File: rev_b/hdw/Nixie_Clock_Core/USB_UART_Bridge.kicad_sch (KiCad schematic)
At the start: 34 parts, among them J1301 USB_B_Mini, U1301 TLV6700, U1302 FT234XD, U1304 TXB0102DCU, U1305 TPD3S014DBVR

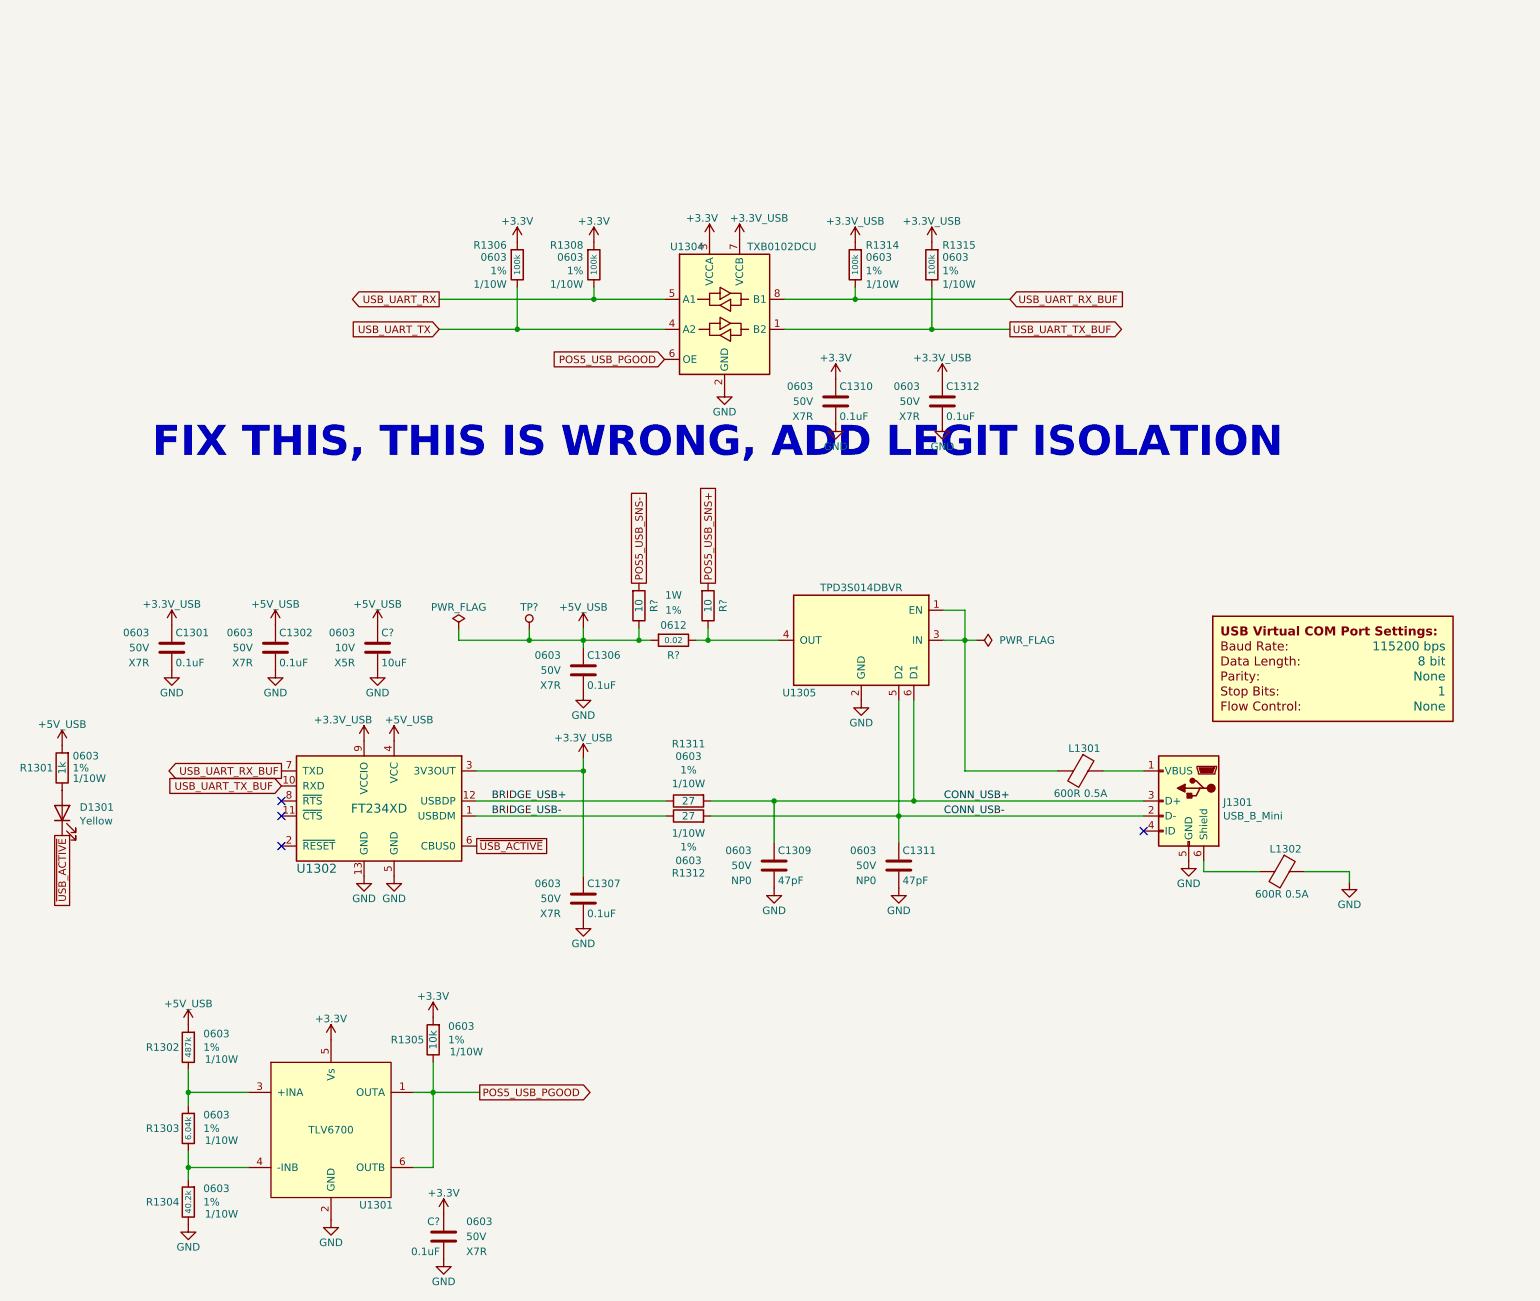
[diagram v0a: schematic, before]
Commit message: lots of rev B control board schematic progress
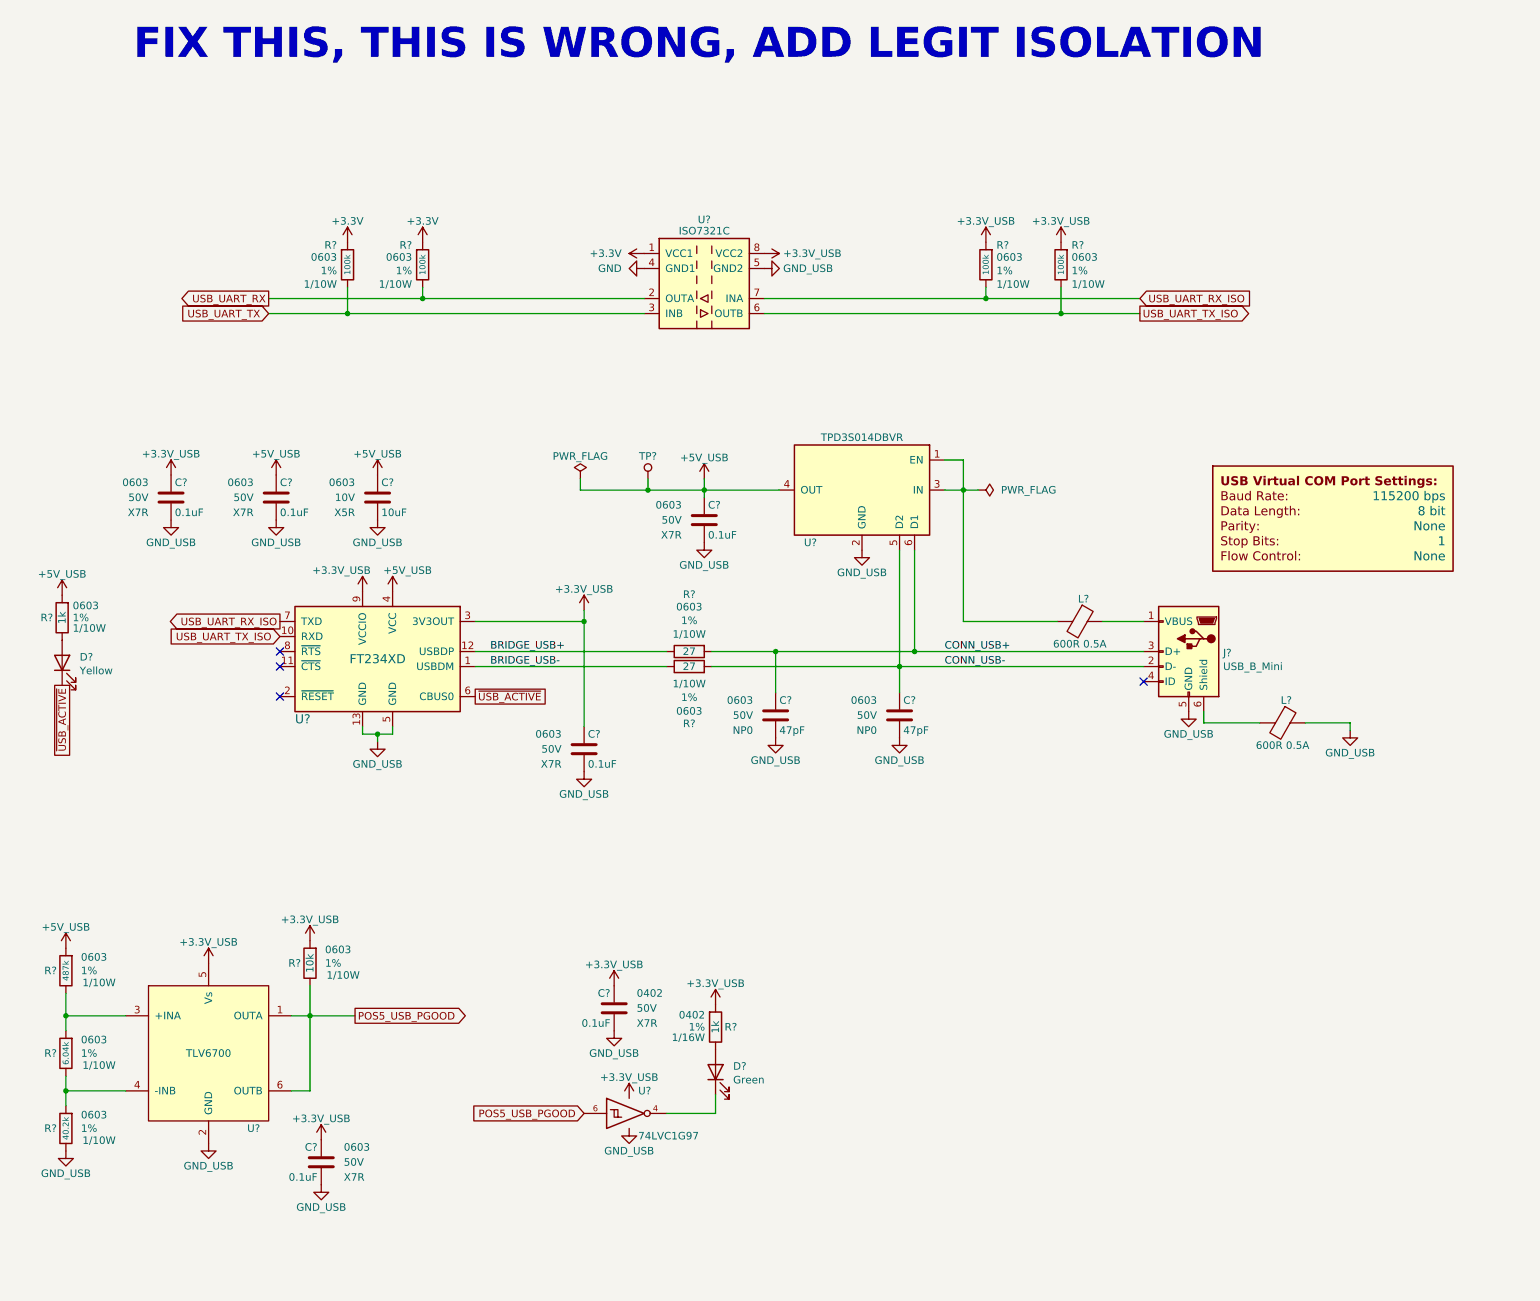
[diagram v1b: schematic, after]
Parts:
- removed C1310, C1312: 0.1uF, Capacitors_SMD:C_0603, symbol Custom_Library:C_Custom
- removed R? (x2): 10, Resistors_SMD:R_0603, symbol Custom_Library:R_Custom
- removed R?: 0.02, Resistors_SMD:R_0612, symbol Custom_Library:R_Custom
- removed U1304: TXB0102DCU, Package_SO:VSSOP-8_2.4x2.1mm_P0.5mm, symbol Logic_LevelTranslator:TXB0102DCU
- added C?: 0.1uF, Capacitors_SMD:C_0402, symbol Custom_Library:C_Custom
- added D?: Green, LEDs:LED_0402, symbol Device:LED
- added R?: 1k, Resistors_SMD:R_0402, symbol Custom_Library:R_Custom
- added U?: 74LVC1G97, Package_TO_SOT_SMD:SOT-363_SC-70-6, symbol Custom Library:74LVC1G97_Power_NOT
- added U?: ISO7321C, Package_SO:SOIC-8_3.9x4.9mm_P1.27mm, symbol Isolator:ISO7321C
- renumbered C1307 to C?, C1309 to C?, C1311 to C?, C1302 to C?, C1306 to C?, C1301 to C?, D1301 to D?, DOC1301 to DOC?, J1301 to J?, L1301 to L?, L1302 to L?, R1314 to R?, R1312 to R?, R1302 to R?, R1311 to R?, R1305 to R?, R1315 to R?, R1304 to R?, R1301 to R?, R1306 to R?, R1303 to R?, R1308 to R?, U1302 to U?, U1301 to U?, U1305 to U?
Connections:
- net +3.3V: now also U?.1 (VCC1); no longer C?.1, R?.1, U?.5 (Vs)
- net +3.3V_USB: now also C?.1, R?.1, U?.5 (Vs), C?.1, R?.1, U?.1 (VCC), U?.5 (VCC), U?.8 (VCC2)
- net +5V_USB: now also U?.4 (OUT)
- net GND: now also U?.4 (GND1); no longer C?.2, C?.2, C?.2, C?.2, C?.2, C?.2, C?.2, C?.2, J?.5 (GND), L?.1, R?.2, U?.13 (GND), U?.2 (GND), U?.2 (GND), U?.5 (GND)
- net POS5_USB_PGOOD: now also U?.6
- net USB_UART_RX: now also U?.2 (OUTA)
- net USB_UART_TX: now also U?.3 (INB)
- net USB_UART_RX_BUF renamed USB_UART_RX_ISO
- net USB_UART_RX_ISO: now also U?.7 (INA)
- net USB_UART_TX_BUF renamed USB_UART_TX_ISO
- net USB_UART_TX_ISO: now also U?.6 (OUTB)
- new net: D?.1 (K), U?.4
- new net: D?.2 (A), R?.2
- new net GND_USB: C?.2, C?.2, C?.2, C?.2, C?.2, C?.2, C?.2, C?.2, C?.2, J?.5 (GND), L?.1, R?.2, U?.13 (GND), U?.2 (GND), U?.2 (GND), U?.2 (GND), U?.3 (GND), U?.5 (GND), U?.5 (GND2)
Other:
- moved on the sheet: C?, D?, J?, L?, R?, TP?, U?

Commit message: more rev b sch progress
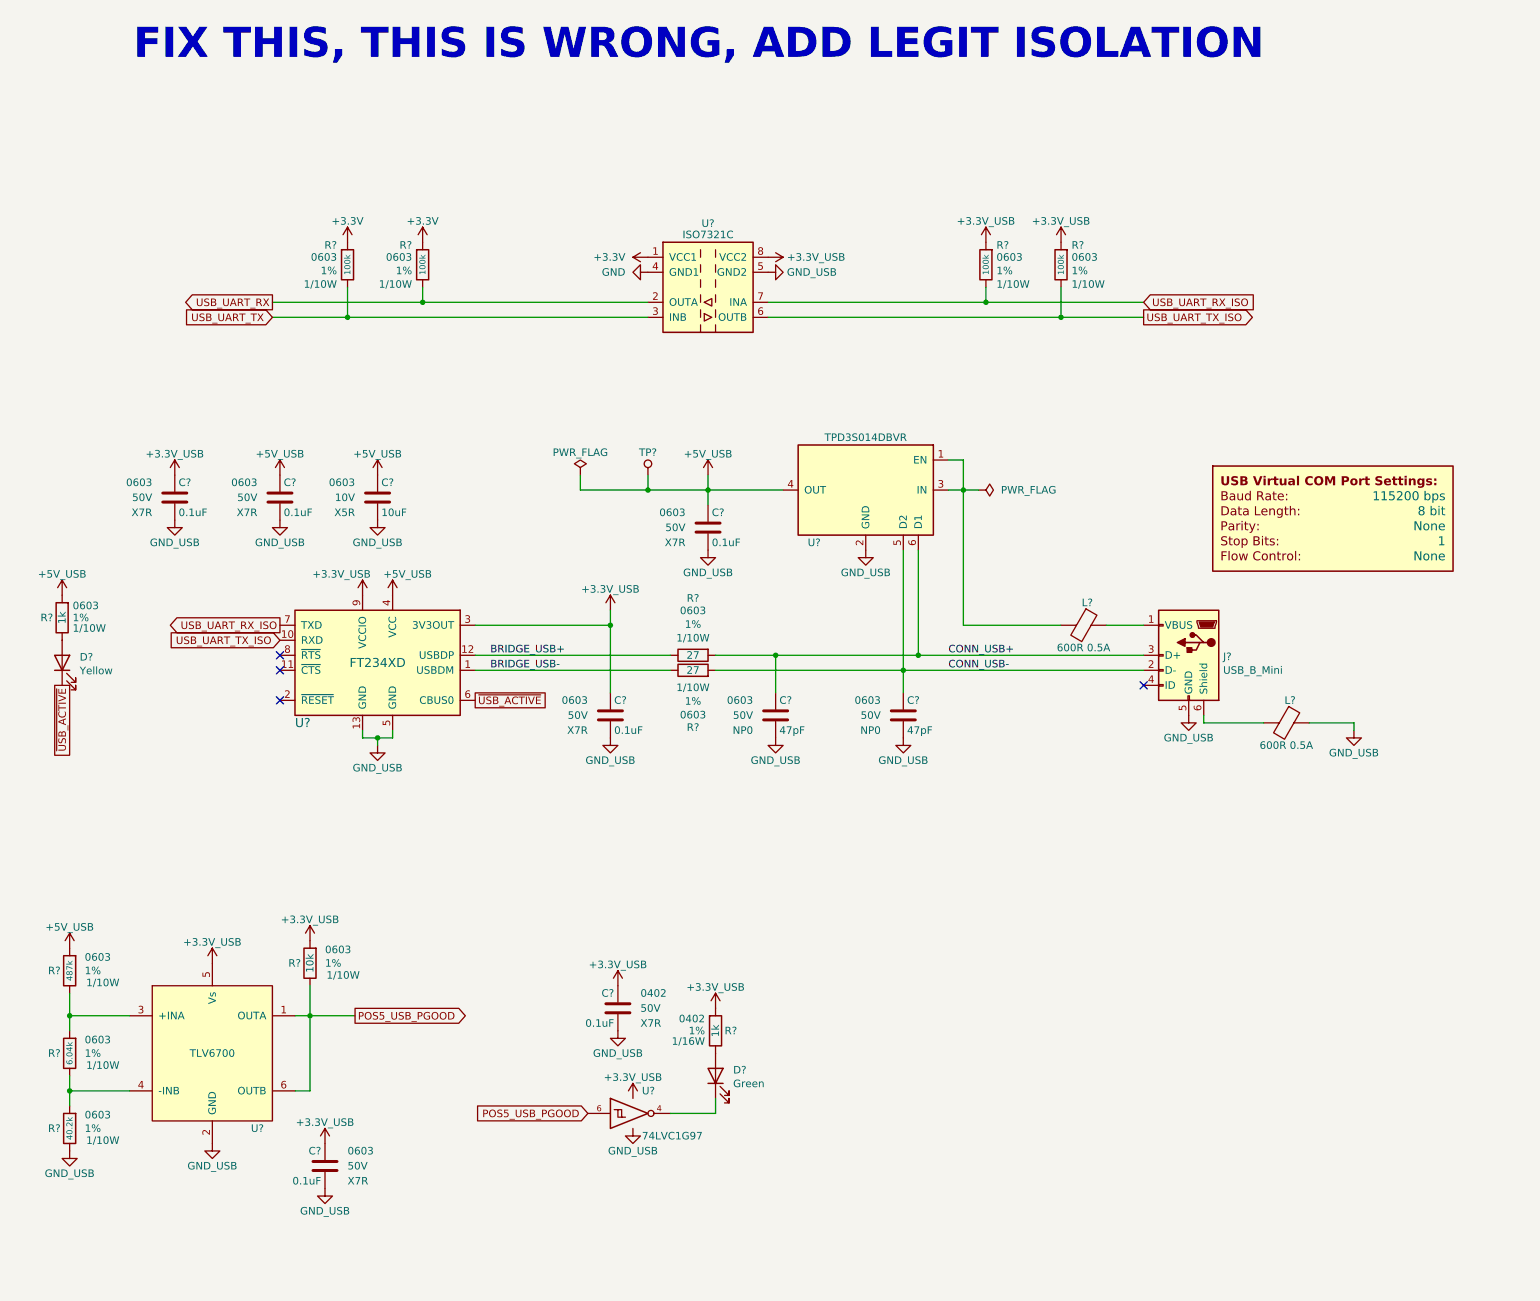
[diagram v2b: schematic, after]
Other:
- moved on the sheet: C?, D?, J?, L?, R?, TP?, U?
